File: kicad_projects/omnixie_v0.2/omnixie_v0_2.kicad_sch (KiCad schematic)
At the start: 67 parts, among them J1 Conn_01x10, J2 SM04B-SRSS-TB, J3 SM04B-SRSS-TB, J4 USB4105-GF-A, J5 Conn_01x04, J6 Conn_01x02, J8 IL-WX-16S-VF-B-E1000E, Q0 BSS123, Q1 BSS123, Q10 BSS123, Q11 BSS123, Q12 IPN50R1K4CEATMA1, Q2 BSS123, Q3 BSS123, Q4 BSS123, Q5 BSS123, Q6 BSS123, Q7 BSS123, Q8 BSS123, Q9 BSS123, T1 ATB322515-0110, U1 CH32V003F4U6, U3 PI4IOE5V6416ZDEX, U4 XC6206P332MR

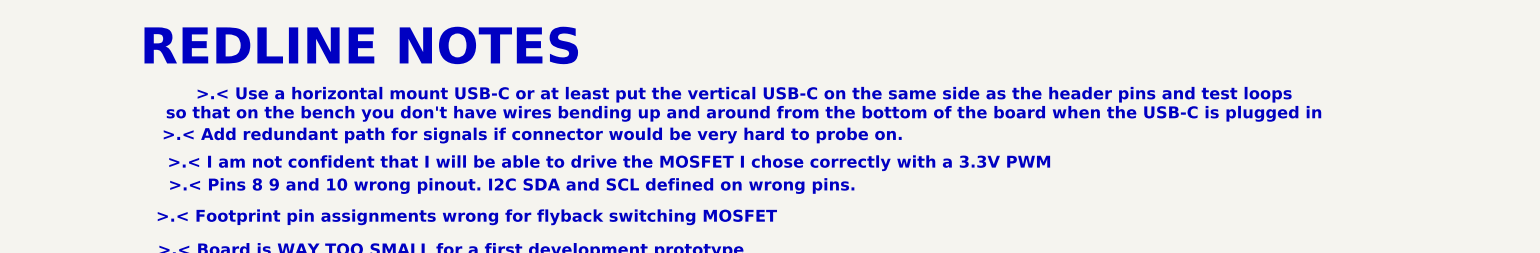
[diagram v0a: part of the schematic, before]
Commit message: new folders for next versions
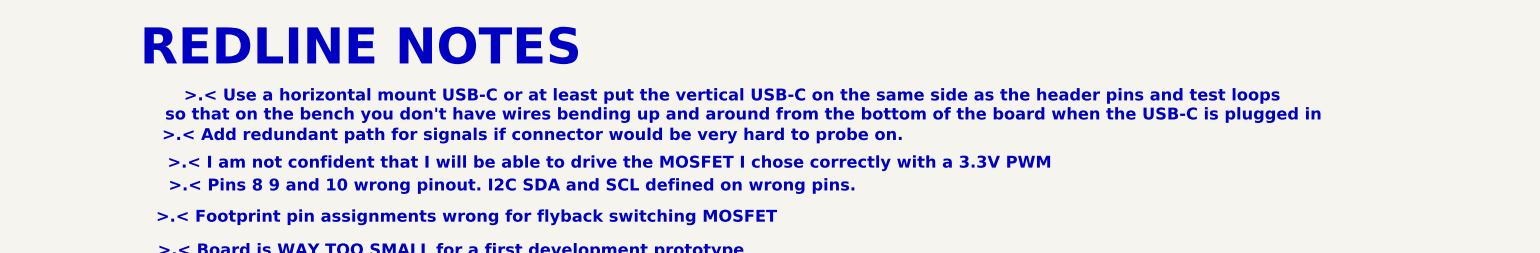
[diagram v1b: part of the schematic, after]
